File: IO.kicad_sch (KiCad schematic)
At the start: 3 parts

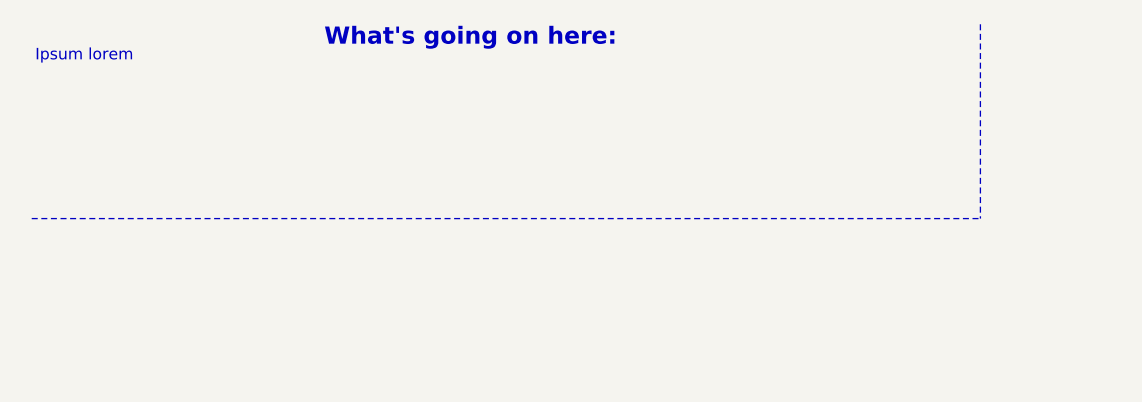
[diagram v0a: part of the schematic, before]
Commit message: added everything to repo
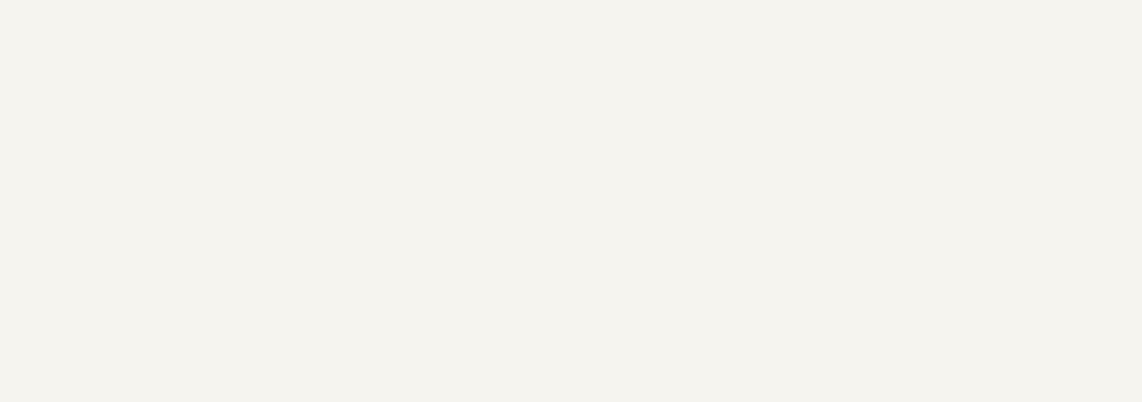
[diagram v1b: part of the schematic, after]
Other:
- note removed: "Ipsum lorem"
- note removed: "What's going on here:"
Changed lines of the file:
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@@
-		)
-	)
-	(text "Ipsum lorem\n"
-		(exclude_from_sim no)
-		(at 18.542 16.256 0)
-		(effects
-			(font
-				(size 1.27 1.27)
-				(color 132 0 0 1)
-			)
-		)
-	)
-	(text "What's going on here:\n"
-		(exclude_from_sim no)
-		(at 61.468 14.224 0)
-		(effects
-			(font
-				(size 1.905 1.905)
-				(thickness 0.381)
-				(bold yes)
-				(color 132 0 0 1)
-			)
 		)
 	)
@@
 		)
 	)
-	(polyline
-		(pts
-			(xy 12.7 34.29) (xy 118.11 34.29)
-		)
-		(stroke
-			(width 0)
-			(type dash)
-			(color 132 0 0 1)
-		)
-	)
 	(wire
 		(pts
@@
 		)
 	)
-	(polyline
-		(pts
-			(xy 118.11 12.7) (xy 118.11 34.29)
-		)
-		(stroke
-			(width 0)
-			(type dash)
-			(color 132 0 0 1)
-		)
-	)
